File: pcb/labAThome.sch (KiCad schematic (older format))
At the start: 109 parts, among them J1 I2C, J11 24.5.GND.3, J12 NEOPIXEL, J13 Power Input 1, J14 Conn_Coaxial, J15 WS2812_OUT, J16 HCP, J2 SRVx, J3 5V, J4 EXT, J5 VPS, J6 FAN2, J7 1wire, J8 1wire, J9 FAN1, K1 G5V-2, K2 G5V-2, K3 G5V-2, M3 SN65HVD230_MODULE, Q1 BC847, Q2 IRLZ44N, Q3 IRLML6344, Q4 BC847, Q5 IRF530, Q6 IRLML5203, SW1 RED, SW2 GREEN, SW4 BLUE, SW5 WHITE, SW7 ROTENC, U1 SR602, U10 MAX3485_MODULE, U11 AM312, U12 24V->4V, U13 LM358, U14 MS4525DO, U15 CCS811_MODULE, U16 24V->5V, U17 DS18B20, U2 TPS5430DDA, U3 Power Input 2, U4 ESP32_DEVKITC_COMPATIBLE, U6 GY-302, U7 Display, U8 MIC, U9 RFM95W-868S2, X1 FAN_6024, m1 Attribution

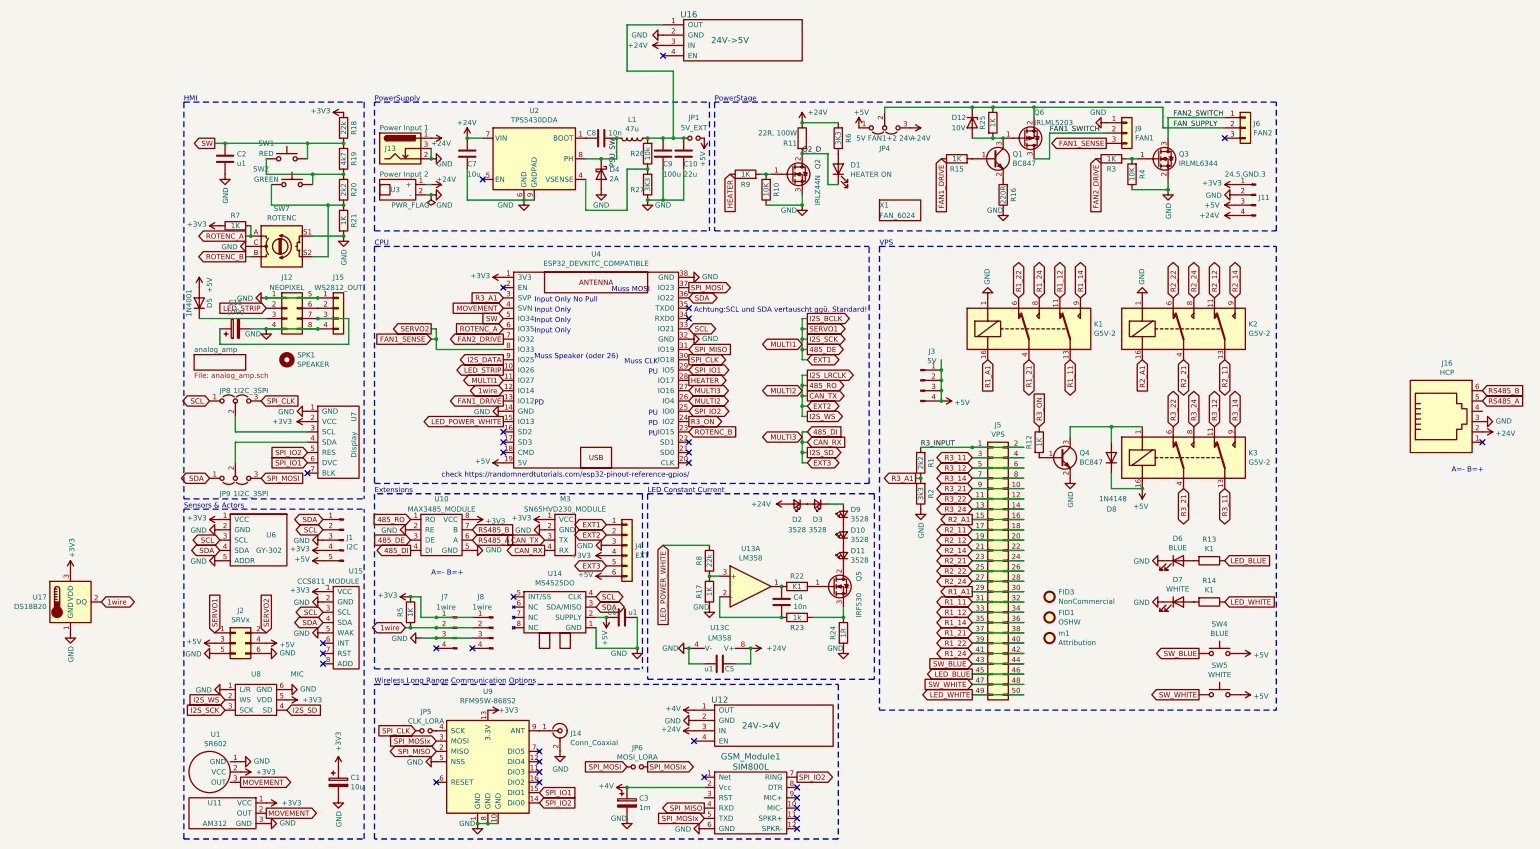
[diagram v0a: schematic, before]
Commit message: pcb V10 as ordered at JLCPCB
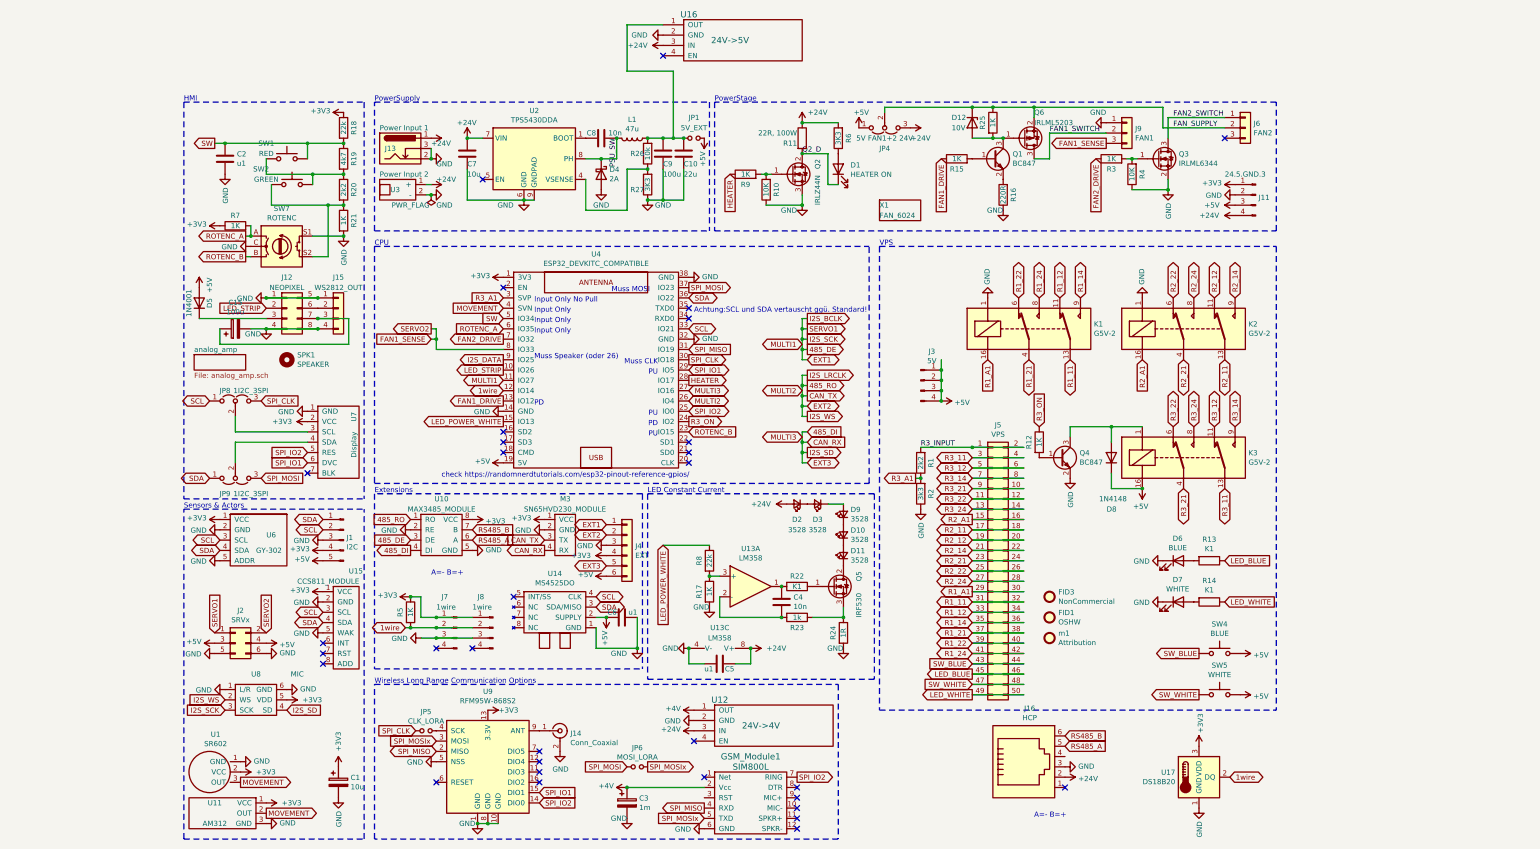
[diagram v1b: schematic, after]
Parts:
- R11: footprint smopla:Resistor_100W -> liebler_PASSIVES:Resistor_100W
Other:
- moved on the sheet: J16, U17
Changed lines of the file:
@@
 F 0 "R11" H 6500 900 50  0000 R CNN
 F 1 "22R, 100W" H 6500 1000 50  0000 R CNN
-F 2 "smopla:Resistor_100W" V 6480 950 50  0001 C CNN
+F 2 "liebler_PASSIVES:Resistor_100W" V 6480 950 50  0001 C CNN
 F 3 "~" H 6550 950 50  0001 C CNN
 F 4 "Heater only" H 6550 950 50  0001 C CNN "Option"
@@
 L Sensor_Temperature:DS18B20 U17
 U 1 1 608FDFE2
-P -550 5450
-F 0 "U17" H -780 5496 50  0000 R CNN
-F 1 "DS18B20" H -780 5405 50  0000 R CNN
-F 2 "Package_TO_SOT_THT:TO-92_Inline" H -1550 5200 50  0001 C CNN
-F 3 "http://datasheets.maximintegrated.com/en/ds/DS18B20.pdf" H -700 5700 50  0001 C CNN
-	1    -550 5450
+P 10400 7150
+F 0 "U17" H 10170 7196 50  0000 R CNN
+F 1 "DS18B20" H 10170 7105 50  0000 R CNN
+F 2 "Package_TO_SOT_THT:TO-92_Inline" H 9400 6900 50  0001 C CNN
+F 3 "http://datasheets.maximintegrated.com/en/ds/DS18B20.pdf" H 10250 7400 50  0001 C CNN
+	1    10400 7150
 	1    0    0    -1
 $EndComp
@@
 L power:+3V3 #PWR066
 U 1 1 6090245F
-P -550 5150
-F 0 "#PWR066" H -550 5000 50  0001 C CNN
-F 1 "+3V3" V -535 5278 50  0000 L CNN
-F 2 "" H -550 5150 50  0001 C CNN
-F 3 "" H -550 5150 50  0001 C CNN
-	1    -550 5150
+P 10400 6850
+F 0 "#PWR066" H 10400 6700 50  0001 C CNN
+F 1 "+3V3" V 10415 6978 50  0000 L CNN
+F 2 "" H 10400 6850 50  0001 C CNN
+F 3 "" H 10400 6850 50  0001 C CNN
+	1    10400 6850
 	1    0    0    -1
 $EndComp
@@
 L power:GND #PWR067
 U 1 1 609030A4
-P -550 5750
-F 0 "#PWR067" H -550 5500 50  0001 C CNN
-F 1 "GND" V -545 5622 50  0000 R CNN
-F 2 "" H -550 5750 50  0001 C CNN
-F 3 "" H -550 5750 50  0001 C CNN
-	1    -550 5750
+P 10400 7450
+F 0 "#PWR067" H 10400 7200 50  0001 C CNN
+F 1 "GND" V 10405 7322 50  0000 R CNN
+F 2 "" H 10400 7450 50  0001 C CNN
+F 3 "" H 10400 7450 50  0001 C CNN
+	1    10400 7450
 	1    0    0    -1
 $EndComp
-Text GLabel -250 5450 2    50   BiDi ~ 0
+Text GLabel 10700 7150 2    50   BiDi ~ 0
 1wire
 $Sheet
@@
 L Connector:6P6C J16
 U 1 1 610E3B2A
-P 12750 3700
-F 0 "J16" H 12807 4267 50  0000 C CNN
-F 1 "HCP" H 12807 4176 50  0000 C CNN
-F 2 "liebler_CONN:WR_MJ_Modular_Jack_Vertical_Plastic_6P6C" V 12750 3725 50  0001 C CNN
-F 3 "~" V 12750 3725 50  0001 C CNN
-F 4 "HörmannGarage only" H 12750 3700 50  0001 C CNN "Option"
-	1    12750 3700
+P 8700 7050
+F 0 "J16" H 8757 7617 50  0000 C CNN
+F 1 "HCP" H 8757 7526 50  0000 C CNN
+F 2 "liebler_CONN:WR_MJ_Modular_Jack_Vertical_Plastic_6P6C" V 8700 7075 50  0001 C CNN
+F 3 "~" V 8700 7075 50  0001 C CNN
+F 4 "HörmannGarage only" H 8700 7050 50  0001 C CNN "Option"
+	1    8700 7050
 	1    0    0    -1
 $EndComp
 Text Notes 2950 5200 0    50   ~ 0
 A=- B=+
-NoConn ~ 13150 3900
+NoConn ~ 9100 7250
 $Comp
 L power:+24V #PWR0106
 U 1 1 6110EDB7
-P 13150 3800
-F 0 "#PWR0106" H 13150 3650 50  0001 C CNN
-F 1 "+24V" V 13165 3928 50  0000 L CNN
-F 2 "" H 13150 3800 50  0001 C CNN
-F 3 "" H 13150 3800 50  0001 C CNN
-	1    13150 3800
+P 9100 7150
+F 0 "#PWR0106" H 9100 7000 50  0001 C CNN
+F 1 "+24V" V 9115 7278 50  0000 L CNN
+F 2 "" H 9100 7150 50  0001 C CNN
+F 3 "" H 9100 7150 50  0001 C CNN
+	1    9100 7150
 	0    1    1    0
 $EndComp
@@
 L power:GND #PWR0107
 U 1 1 6110F531
-P 13150 3700
-F 0 "#PWR0107" H 13150 3450 50  0001 C CNN
-F 1 "GND" V 13155 3572 50  0000 R CNN
-F 2 "" H 13150 3700 50  0001 C CNN
-F 3 "" H 13150 3700 50  0001 C CNN
-	1    13150 3700
+P 9100 7050
+F 0 "#PWR0107" H 9100 6800 50  0001 C CNN
+F 1 "GND" V 9105 6922 50  0000 R CNN
+F 2 "" H 9100 7050 50  0001 C CNN
+F 3 "" H 9100 7050 50  0001 C CNN
+	1    9100 7050
 	0    -1   -1   0
 $EndComp
-Text GLabel 13150 3500 2    50   Input ~ 0
+Text GLabel 9100 6850 2    50   Input ~ 0
 RS485_A
-Text GLabel 13150 3400 2    50   Input ~ 0
+Text GLabel 9100 6750 2    50   Input ~ 0
 RS485_B
-Text Notes 12850 4200 0    50   ~ 0
+Text Notes 8800 7550 0    50   ~ 0
 A=- B=+
 Text GLabel 3350 4850 2    50   Input ~ 0
